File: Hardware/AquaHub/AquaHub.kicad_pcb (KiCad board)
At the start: 2 copper layers, 192 x 112 mm, 76 parts, among them J1 Screw_Terminal_01x02, J10 PinHeader6, J13 PinHeader2, J14 PinHeader3, J2 Screw_Terminal_01x02, J3 Screw_Terminal_01x02, J4 Screw_Terminal_01x02, J5 Screw_Terminal_01x02, J6 Screw_Terminal_01x02, J7 Screw_Terminal_01x02, J8 Conn_01x15_Female, K1 5A Relay, K2 5A Relay, K3 5A Relay, K4 5A Relay, K5 5A Relay, K6 5A Relay, Q2 2SC1815, SW7 Reset, U1 ESP32-WROOM, U2 Current Sense, U3 1A 3.3V, U4 Low-Side Driver, U5 1A 5V, U6 TCA9534, U7 DS1307+, U8 TPIC2810D, Y1 32.768KHz

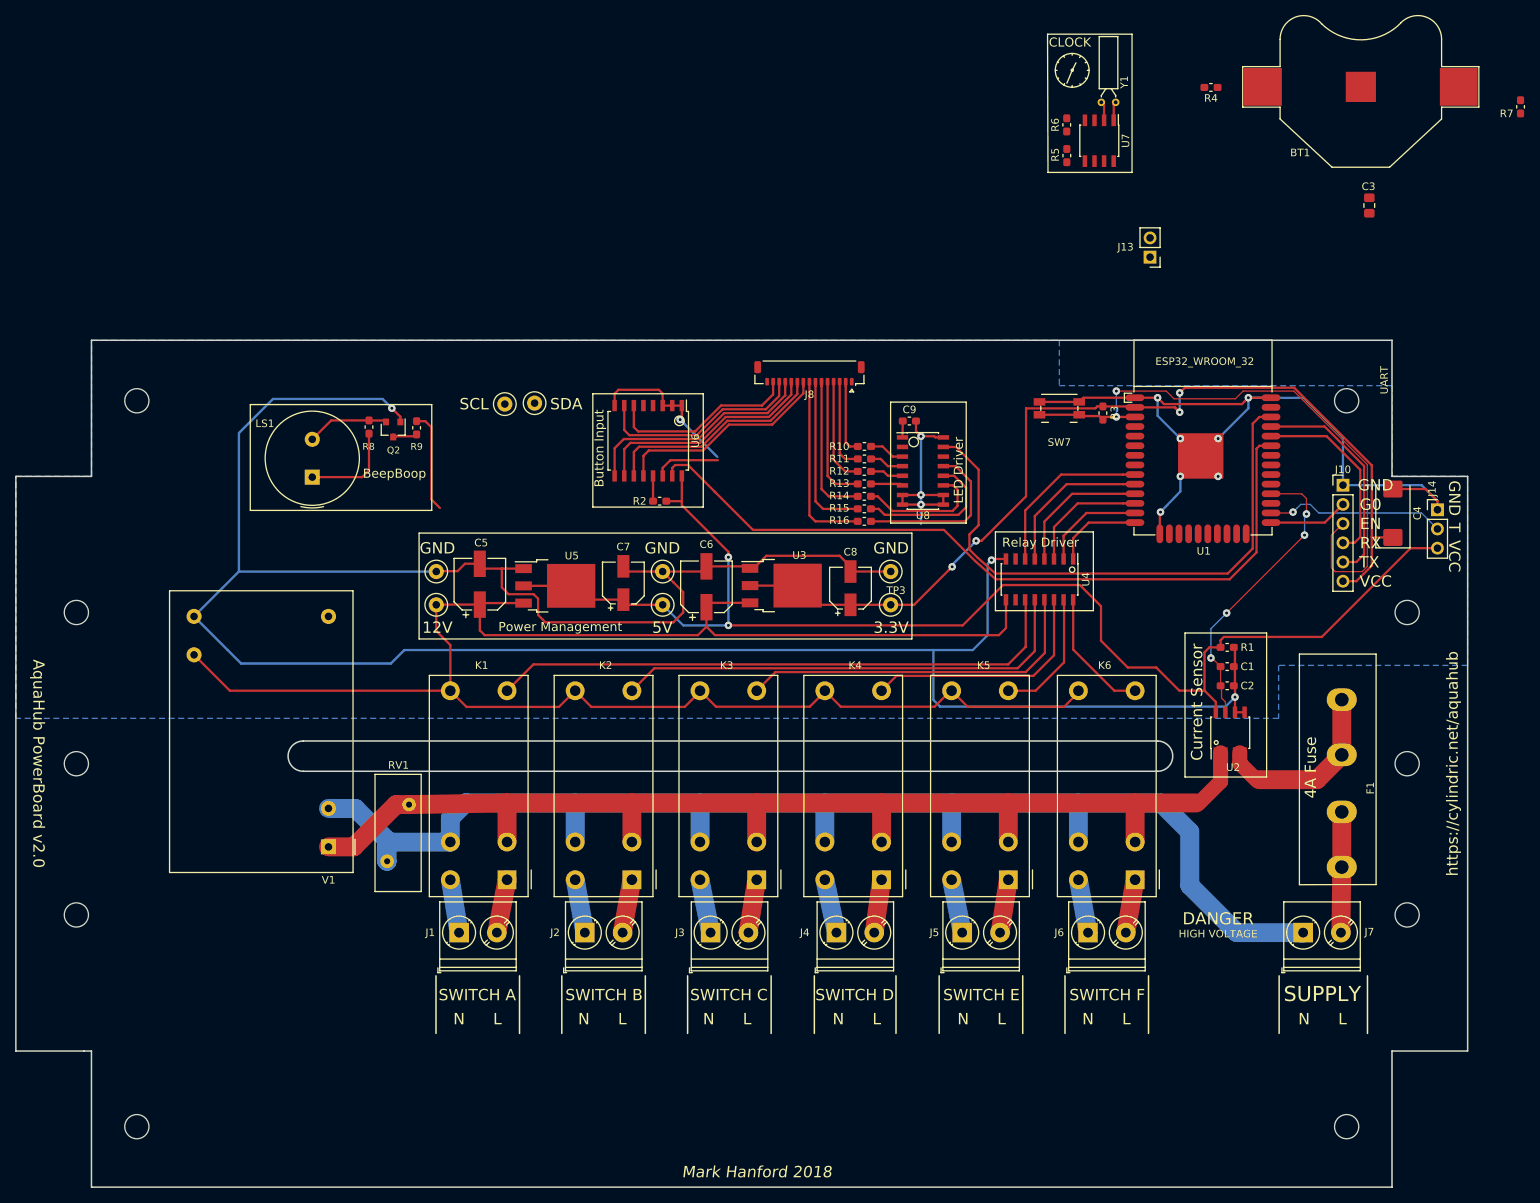
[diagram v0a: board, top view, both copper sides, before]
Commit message: Finalising the Rev2 hardware.
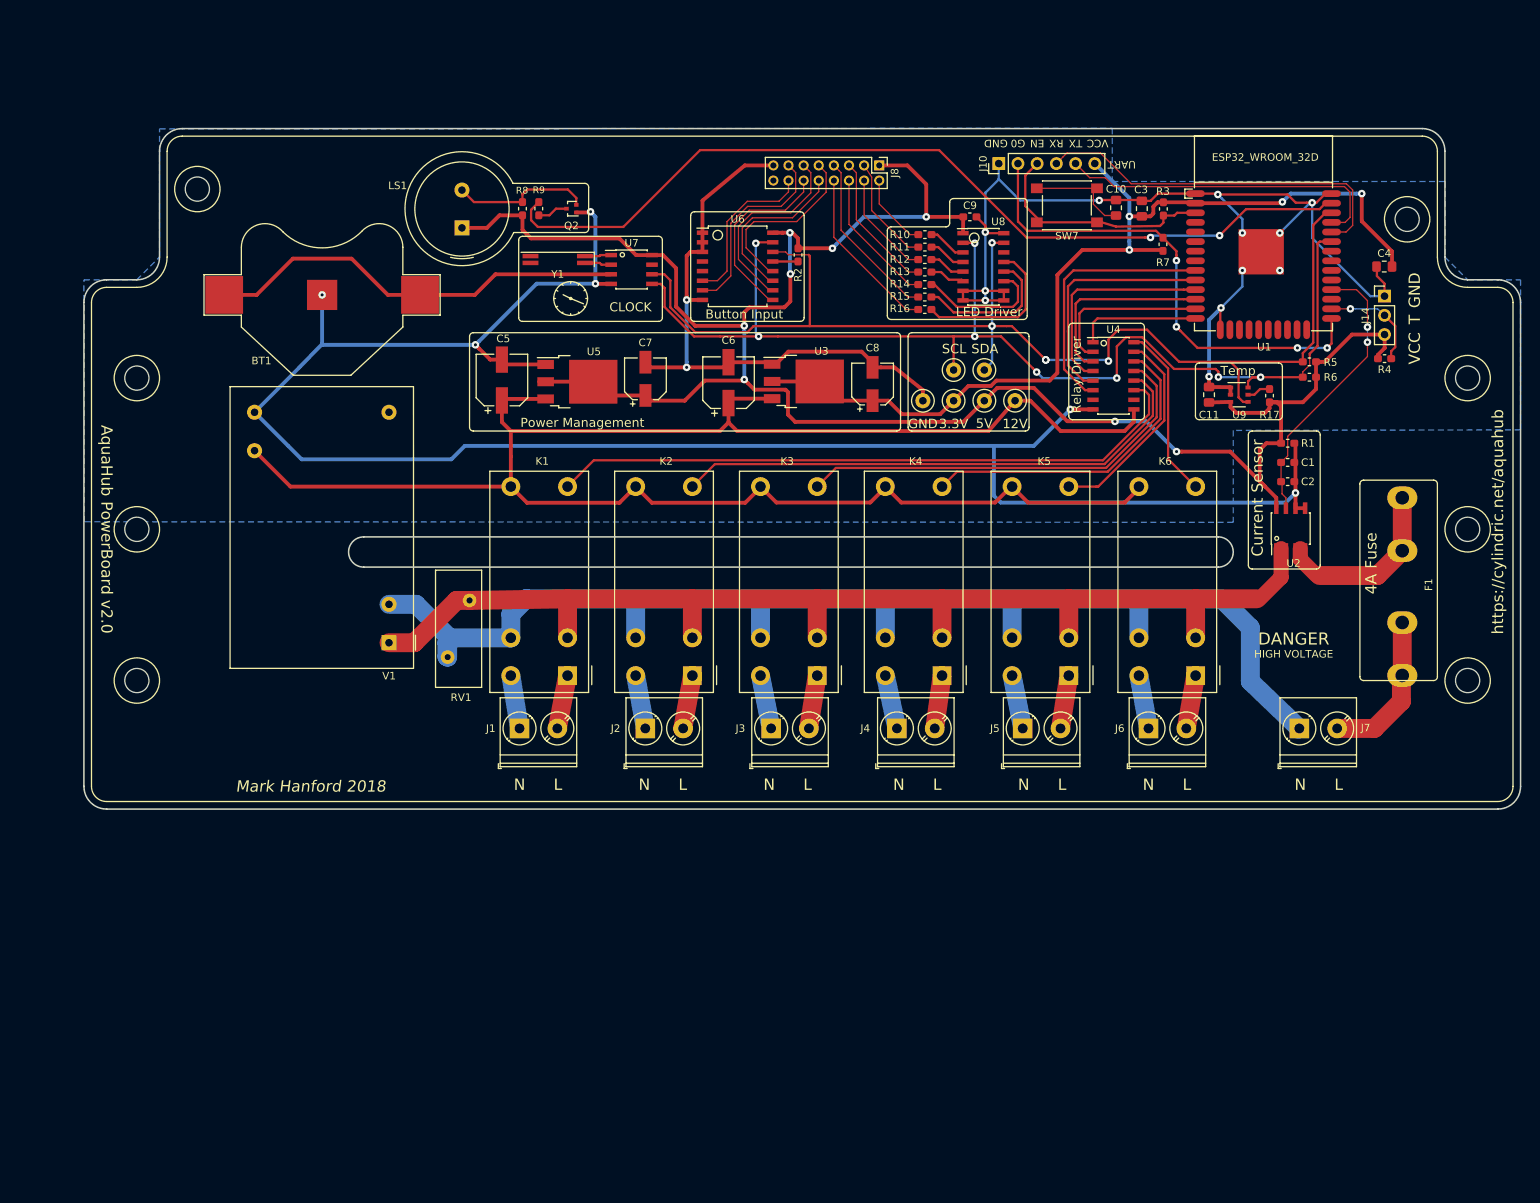
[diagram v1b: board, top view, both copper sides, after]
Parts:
- removed H10, H9: MountingHole, MountingHole:MountingHole_3.2mm_M3
- removed J13: PinHeader2, Connector_PinHeader_2.54mm:PinHeader_1x02_P2.54mm_Vertical
- removed TP5: Test_12V_GND, TestPoint:TestPoint_Loop_D2.50mm_Drill1.0mm
- removed TP6: TEST_5V_GND, TestPoint:TestPoint_Loop_D2.50mm_Drill1.0mm
- added C10: 0.1uF, Capacitor_SMD:C_0805_2012Metric_Pad1.15x1.40mm_HandSolder, F.Cu at (189.5, 42.5)
- added C11: 0.1uF, Capacitor_SMD:C_0805_2012Metric_Pad1.15x1.40mm_HandSolder, F.Cu at (201.8, 67.2)
- added R17: 1.5k, Resistor_SMD:R_0603_1608Metric_Pad1.05x0.95mm_HandSolder, F.Cu at (209.8, 67.3)
- added U9: PCT2075, Package_SO:TSOP-6_1.65x3.05mm_P0.95mm, F.Cu at (205.8, 67.2)
- C4: value 100uF -> 0.1uF; footprint Capacitor_Tantalum_SMD:CP_EIA-7343-31_Kemet-D_Pad2.25x2.55mm_HandSolder -> Capacitor_SMD:C_0805_2012Metric_Pad1.15x1.40mm_HandSolder
- F1: footprint AquaFootprints:Fuse_Clip_5mm -> Fuse:Fuseholder_Glass_5mmx20mm
- J8: footprint Connector_Hirose:Hirose_DF52-15S-0.8H_1x15-1MP_P0.80mm_Horizontal -> Connector_PinHeader_2.00mm:PinHeader_2x08_P2.00mm_Vertical
- Q2: value 2SC1815 -> 2SC4738; footprint Package_TO_SOT_SMD:SOT-23 -> Package_TO_SOT_SMD:SOT-416
- SW7: footprint Button_Switch_SMD:Panasonic_EVQPUJ_EVQPUA -> Button_Switch_SMD:SW_SPST_PTS645
- TP1: value TEST_5V -> TEST_5V_GND
- TP3: value Test_3V3_GND -> TEST_5V
- U1: footprint Module:Espressif_ESP32_WROOM_32_SMT -> Module:Espressif_ESP32_WROOM_32D_SMT
- U2: value Current Sense -> MLX91210
- U4: value Low-Side Driver -> TPL7407LADR
- Y1: footprint Crystal:Crystal_C26-LF_D2.1mm_L6.5mm_Horizontal -> Crystal:Crystal_SMD_SeikoEpson_MC146-4Pin_6.7x1.5mm_HandSoldering
- moved H1 206.5 mm to (228.0, 44.0)
- moved BT1 140.1 mm to (84.5, 54.0)
- moved H4 100.3 mm to (236.0, 65.0)
- moved TP4 81.2 mm to (176.1, 68.0)
- moved Y1 76.7 mm to (115.7, 49.3)
- moved U7 64.2 mm to (125.4, 50.6), turned to 0 degrees
- moved TP7 63.6 mm to (172.1, 63.9)
- moved J10 62.3 mm to (174.0, 36.6), turned to 90 degrees
- moved TP8 55.6 mm to (168.0, 63.9)
- moved R7 50.7 mm to (195.7, 47.3)
- moved R6 46.3 mm to (215.1, 64.9), turned to 0 degrees
- moved TP1 43.7 mm to (164.0, 68.0)
- moved R4 42.6 mm to (225.0, 62.4)
- moved R5 42.1 mm to (215.1, 62.9), turned to 180 degrees
- moved LS1 38.5 mm to (103.0, 45.1)
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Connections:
- SW7 pad 2: GND -> Net-(C10-Pad1)
- TP1 pad 1: +5V -> GND
- TP3 pad 1: GND -> +5V
- Y1 pad 2: Net-(U7-Pad2) -> Net-(Y1-Pad2)
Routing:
- net /Sounder: track 13.4 -> 119.9 mm, vias 0 -> 2
- net +5V: track 188.7 -> 278.0 mm, vias 2 -> 8
- net SCL: track 85.1 -> 160.5 mm, vias 0 -> 5
- net +BATT: track 0.00 -> 56.3 mm
- net SDA: track 102.1 -> 157.3 mm, vias 0 -> 8
- net /IO0: track 10.5 -> 65.5 mm, vias 0 -> 4
- net /EN: track 80.1 -> 31.0 mm, vias 2 -> 0
- net /RX: track 25.1 -> 49.6 mm
- net GND: track 511.8 -> 496.7 mm, vias 14 -> 20
- net /TX: track 29.4 -> 43.9 mm
- net Net-(C10-Pad1): track 0.00 -> 13.9 mm
- net /POW1: track 22.9 -> 34.7 mm
- net /POW2: track 20.7 -> 32.0 mm
- net RE5: track 17.2 -> 27.7 mm
- net RE4: track 32.1 -> 42.3 mm
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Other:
- board size 192 x 112 mm -> 190 x 90 mm
- net class Power added: clearance 0.2, trace_width 0.508, via_dia 1, via_drill 0.4
- board text added: "Temp"
- board text removed: "BeepBoop"
- board text removed: "SUPPLY"
- board text removed: "SWITCH A"
- board text removed: "SWITCH B"
- board text removed: "SWITCH C"
- board text removed: "SWITCH D"
- board text removed: "SWITCH E"
- board text removed: "SWITCH F"
